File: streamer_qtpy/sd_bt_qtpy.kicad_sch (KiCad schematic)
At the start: 5 parts, among them J1 Micro_SD_Card_Det, U1 SD_MMC_FOOTPRINT, U2 QTPyESP32

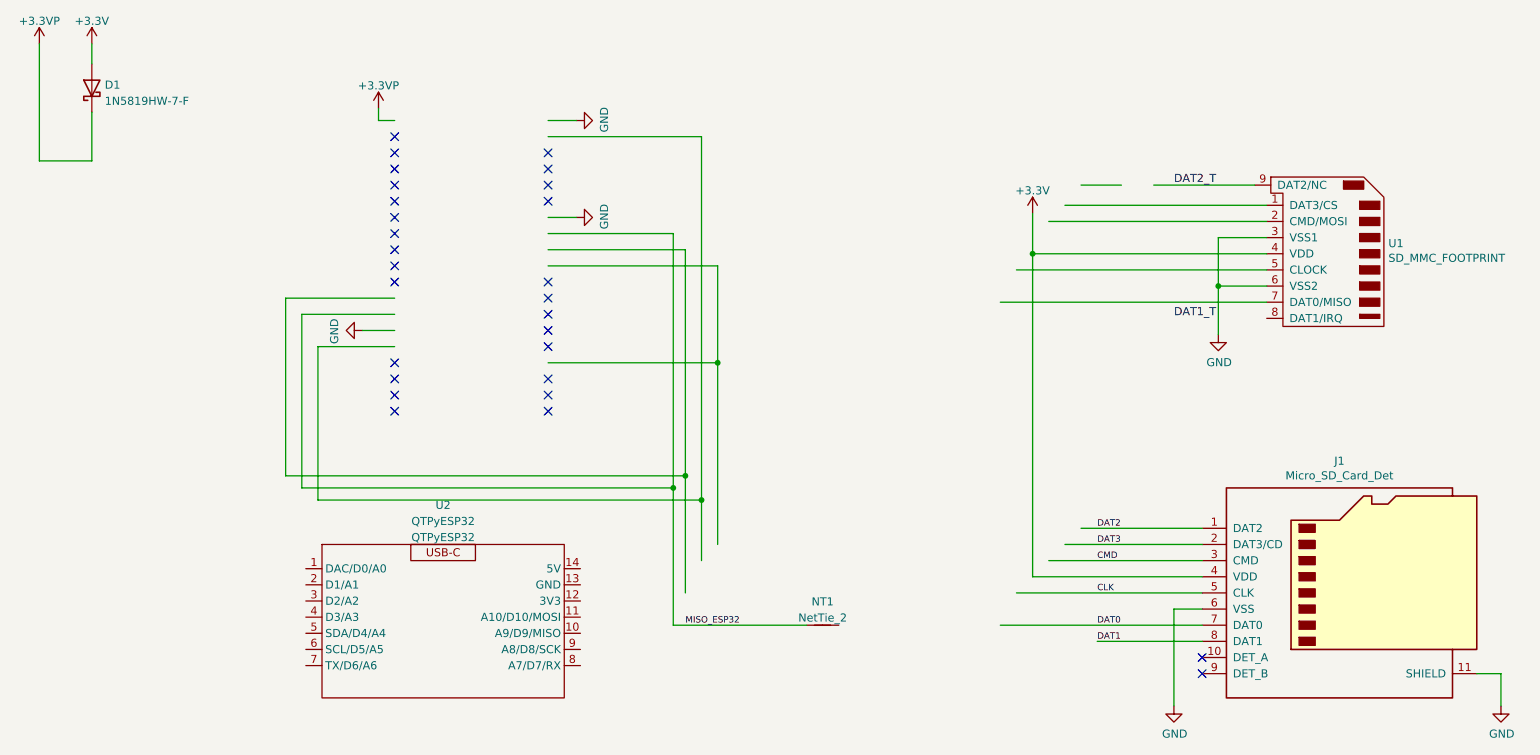
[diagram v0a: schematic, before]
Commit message: ordered from jlcpcb
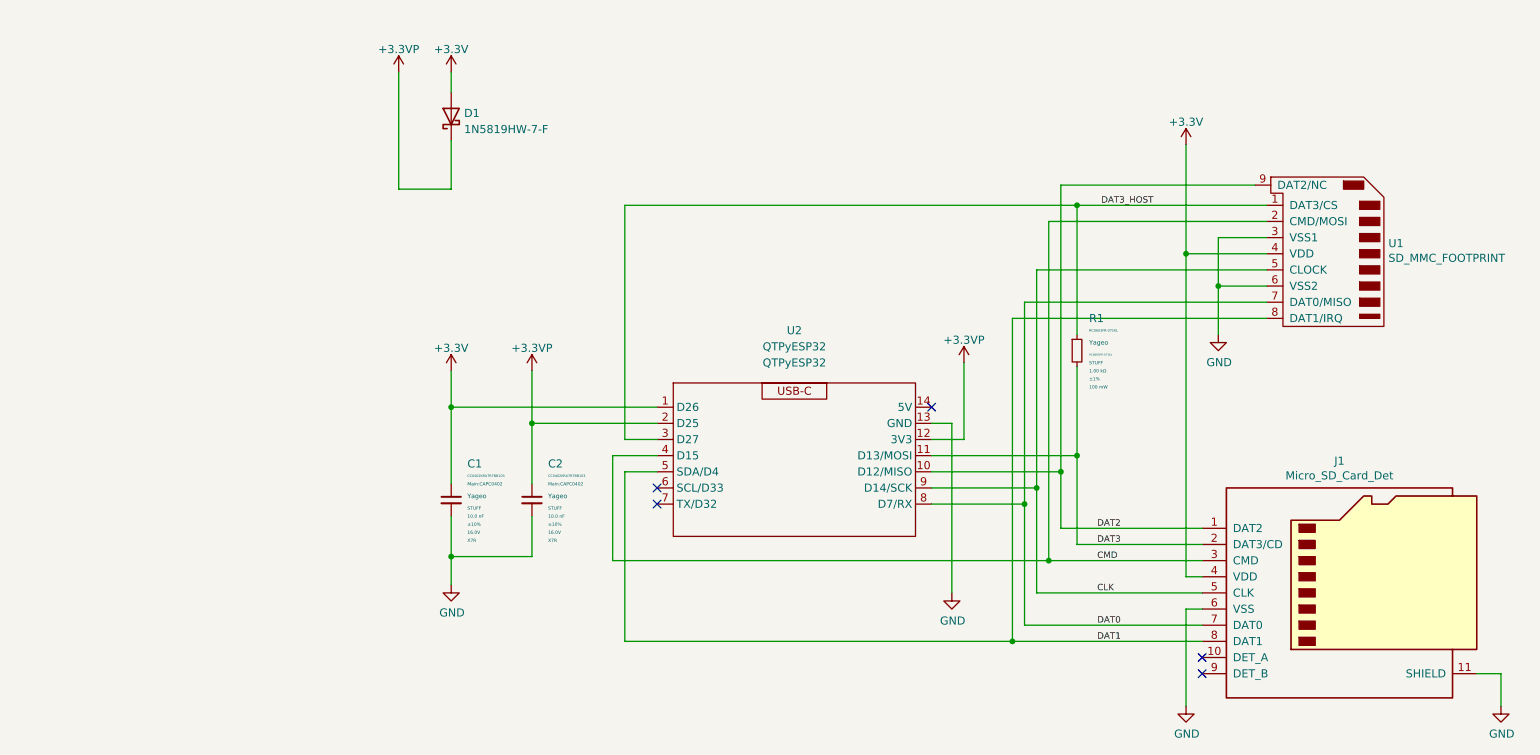
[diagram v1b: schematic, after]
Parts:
- removed NT1: NetTie_2, NetTie:NetTie-2_SMD_Pad0.5mm, symbol Device:NetTie_2
- added C1, C2: CC0402KRX7R7BB103, Main:CAPC0402, symbol cap_smd:CC0402KRX7R7BB103
- added R1: RC0603FR-071KL, Main:RESC0603, symbol res_smd:RC0603FR-071KL
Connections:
- net DAT2_T is gone; now on net DAT2: U1.9 (DAT2/NC)
- net +3.3V: now also U2.1 (D26), C1.1
- net +3.3VP: now also U2.12 (3V3), U2.2 (D25), C2.1
- net CLK: now also U1.5 (CLOCK), U2.9 (D14/SCK)
- net CMD: now also U1.2 (CMD/MOSI), U2.4 (D15)
- net DAT0: now also U1.7 (DAT0/MISO), U2.8 (D7/RX)
- net DAT1: now also U1.8 (DAT1/IRQ), U2.5 (SDA/D4)
- net DAT2: now also U2.10 (D12/MISO)
- net DAT3: now also U2.11 (D13/MOSI), R1.2
- net GND: now also U2.13 (GND), C1.2, C2.2
- net DAT3_HOST: now reaches U1.1 (DAT3/CS)
- net DAT3_HOST: now also U2.3 (D27), R1.1
- no-connect marks 28 -> 5
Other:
- moved on the sheet: D1
